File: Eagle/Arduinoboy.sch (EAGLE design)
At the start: 22 parts

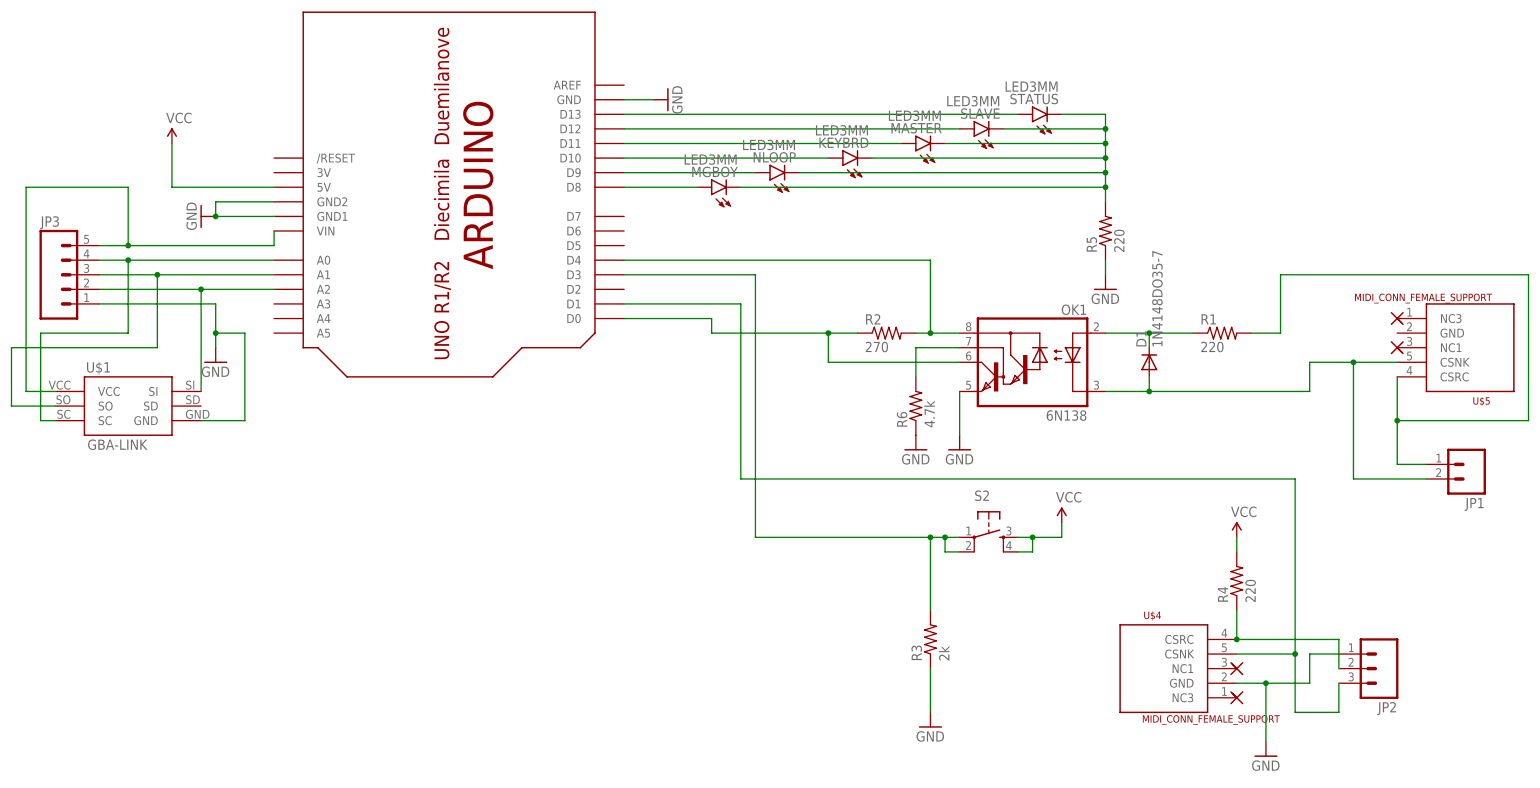
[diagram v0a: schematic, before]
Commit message: Add eagle files for v1.1.0
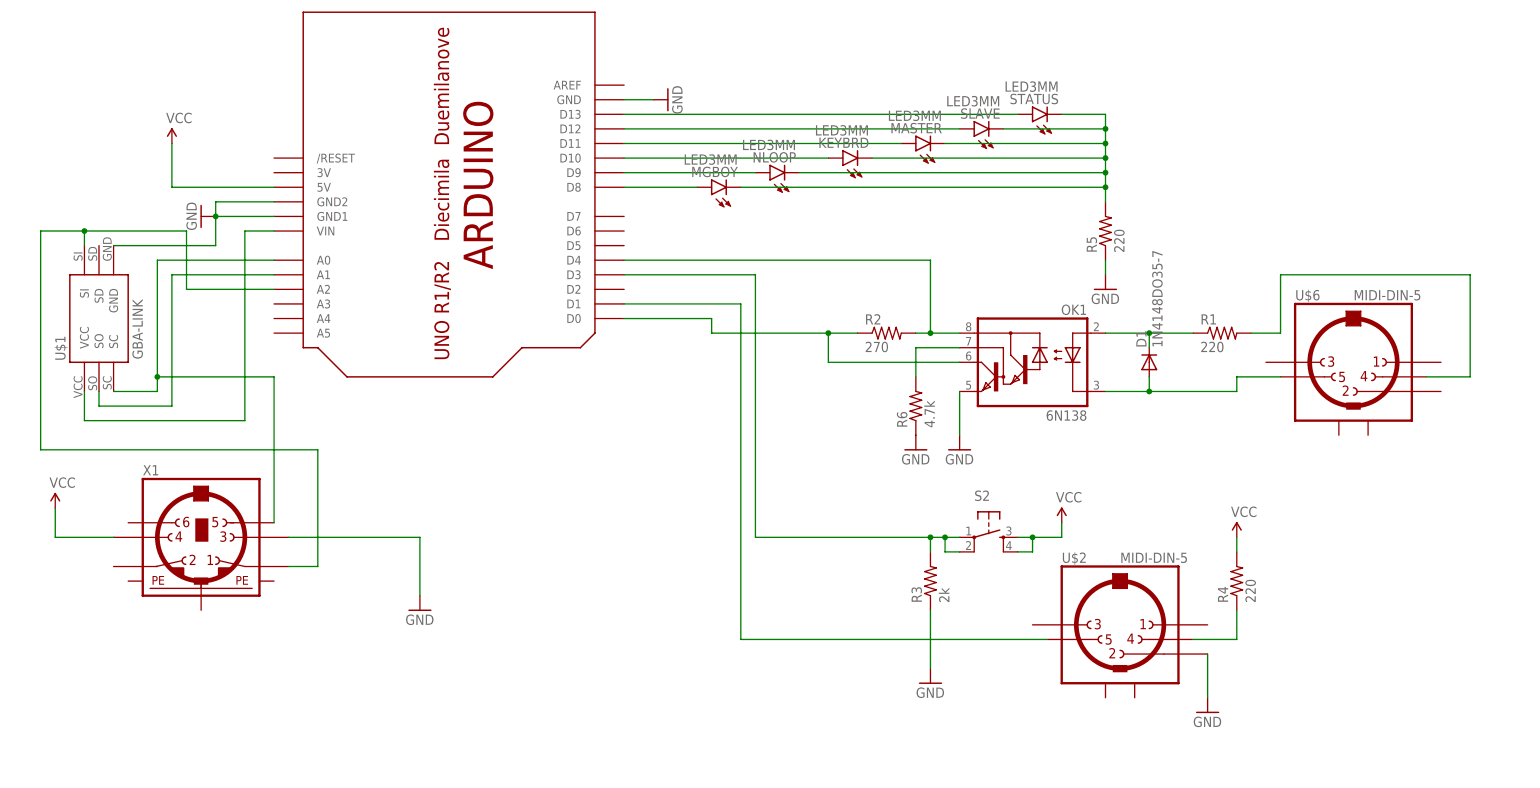
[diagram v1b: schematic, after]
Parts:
- removed JP1: (no value), SparkFun-Connectors:M025MM
- removed JP2: (no value), SparkFun-Connectors:M03-SCREW-5MM
- removed JP3: (no value), SparkFun-Connectors:M05SCREW
- removed U$4, U$5: MIDI_CONN_FEMALE_SUPPORT, SparkFun-Connectors:MIDI_CONN_FEMALE_SUPPORT
- added U$2, U$6: MIDI-DIN-5, MIDI by Jazz:MIDI-DIN-5
- added X1: (no value), mini_din:MINI_DIN_6
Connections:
- removed net N$22: JP3.3, U$1.SO, U$3.A1
- removed net N$23: JP3.2, U$1.SI, U$3.A2
- removed net N$24: JP3.5, U$1.VCC, U$3.VIN
- new net N$19: R1.2, U$6.4
- new net N$20: U$1.SI, U$3.A2, X1.1
- new net N$21: U$1.SO, U$3.A1
- net GND: now also U$2.2, X1.3; no longer JP2.1, JP3.1, U$4.GND
- net N$17: now also X1.5; no longer JP3.4
- net N$18: now also U$1.VCC, U$3.VIN; no longer JP1.1, R1.2, U$5.CSRC
- net N$2: now also U$6.5; no longer JP1.2, U$5.CSNK
- net N$5: now also U$2.4; no longer JP2.2, U$4.CSRC
- net N$7: now also U$2.5; no longer JP2.3, U$4.CSNK
- net VCC: now also X1.4
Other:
- moved on the sheet: R3, U$1
